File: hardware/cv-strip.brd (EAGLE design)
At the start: 140.7 x 40.8 mm, 83 parts, among them IC1 PIC16F1825SO14, IC2 74HC595D, IC3 MCP4728_QUAD_DAC, IC4 LM324D, IC5 REG1117, IC6 74HC595D

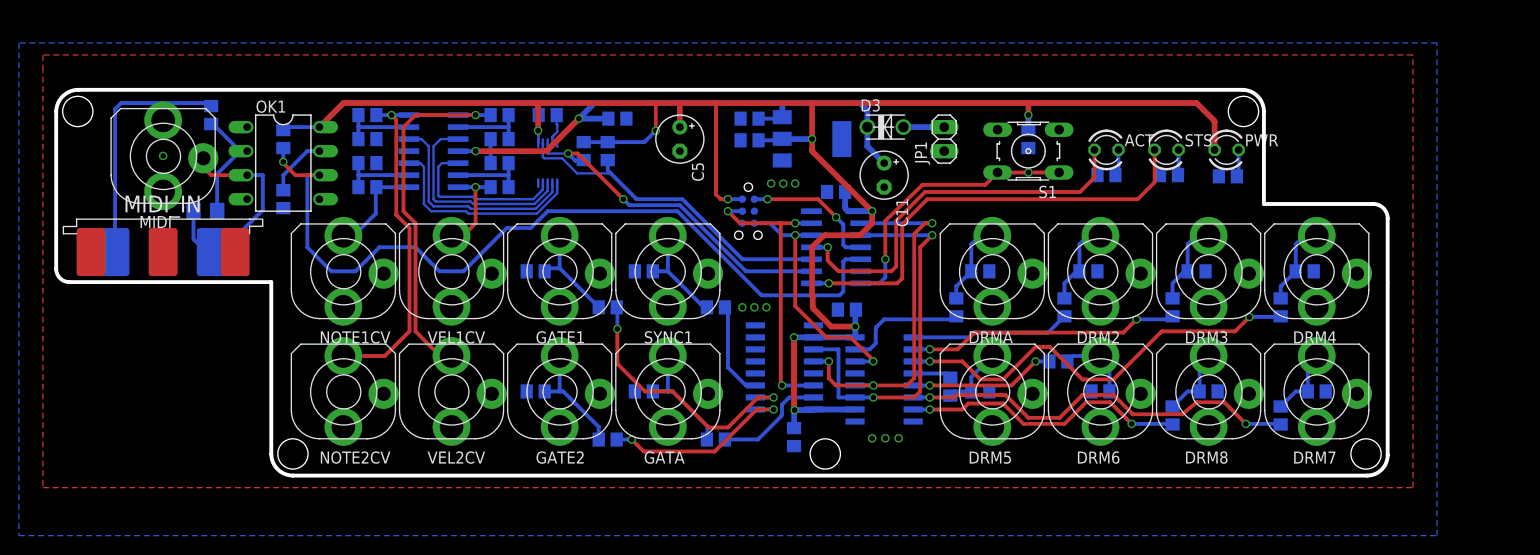
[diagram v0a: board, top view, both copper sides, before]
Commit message: getting there
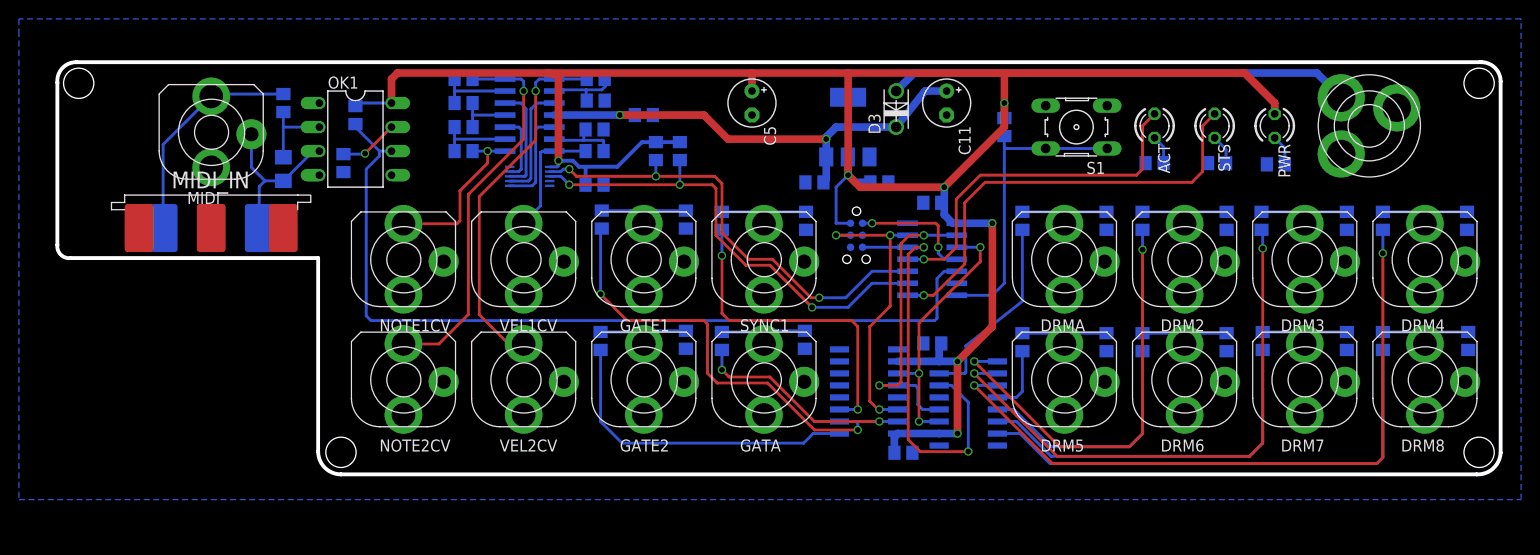
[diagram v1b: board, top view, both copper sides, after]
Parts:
- removed JP1: (no value), pinhead:1X02
- added U$2: PWR_SOCKET_2_1MM, jason_eagle6:PWR_SOCKET_2_1MM
- moved C24 27.9 mm to (149.4, 13.0), turned to 270 degrees
- moved R34 23.6 mm to (140.3, 13.0)
- moved DRM8 22.9 mm to (144.8, 8.89)
- moved C1 18.0 mm to (79.4, 25.7), turned to 270 degrees
- moved C19 18.0 mm to (149.2, 25.7), turned to 270 degrees
- moved C4 17.9 mm to (79.2, 13.1), turned to 270 degrees
- moved C2 16.8 mm to (66.7, 25.8), turned to 270 degrees
- moved C3 16.8 mm to (66.7, 13.1), turned to 270 degrees
- moved C16 16.7 mm to (136.5, 25.7), turned to 270 degrees
- moved C15 15.5 mm to (123.8, 25.7), turned to 270 degrees
- moved C17 14.4 mm to (87.1, 29.7), turned to 0 degrees
- moved C21 14.4 mm to (111.1, 25.7), turned to 270 degrees
- moved C23 14.3 mm to (123.8, 12.8), turned to 270 degrees
- moved C20 14.3 mm to (111.1, 12.8), turned to 270 degrees
- moved R24 14.1 mm to (140.3, 25.7)
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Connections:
- net GND: now also U$2.PIN; no longer JP1.1
- net N$40: now also U$2.BARREL; no longer JP1.2
- net VOUTA: now also IC4.5; no longer IC4.10
- net VOUTB: now also IC4.3; no longer IC4.12
- net VOUTC: now also IC4.12; no longer IC4.3
- net VOUTD: now also IC4.10; no longer IC4.5
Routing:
- net N$40: track 4.32 -> 48.9 mm
- net N$48: track 29.7 -> 59.7 mm
- net N$46: track 16.9 -> 46.1 mm, vias 0 -> 2
- net N$47: track 45.2 -> 73.4 mm
- net N$15: track 10.2 -> 34.5 mm, vias 0 -> 2
- net N$53: track 30.5 -> 53.7 mm, vias 2 -> 0
- net N$16: track 28.5 -> 45.9 mm
- net SR_DAT2: track 26.7 -> 43.9 mm
- net VDD: track 217.3 -> 232.1 mm, vias 9 -> 7
- net N$22: track 36.2 -> 50.1 mm, vias 2 -> 3
- net N$21: track 36.2 -> 49.7 mm, vias 0 -> 3
- net N$13: track 20.9 -> 34.2 mm, vias 2 -> 0
- net SR_CLK: track 41.2 -> 28.0 mm, vias 2 -> 3
- net VOUTA: track 22.2 -> 10.6 mm
- net N$12: track 11.8 -> 22.9 mm, vias 0 -> 2
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- removed copper zone on layer 1, net GND
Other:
- board size 140.7 x 40.8 mm -> 152.5 x 43.6 mm
